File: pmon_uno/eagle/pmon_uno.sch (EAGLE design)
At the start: 42 parts, among them J1 USB, J2 USB, Q1 16Mhz, U1 LTC2943, U2 FT232RL, U3 LT1764AEQ, U4 ATMEGA328TQFP32

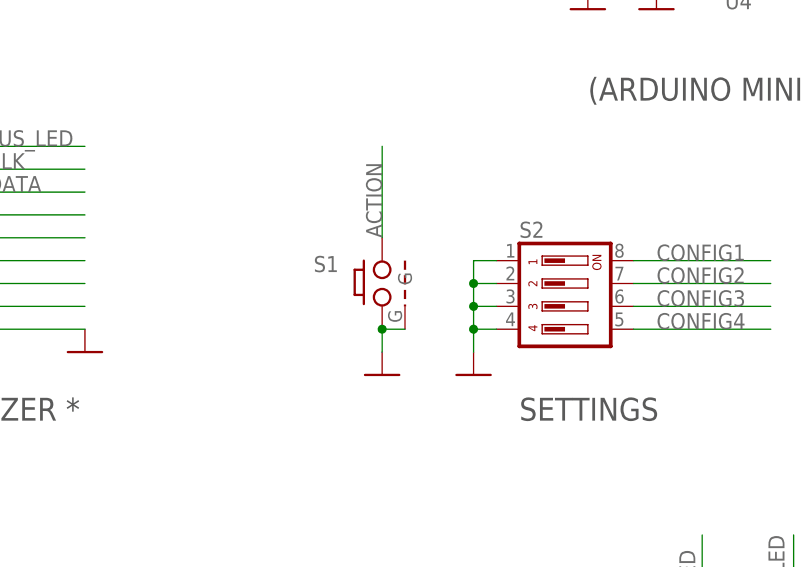
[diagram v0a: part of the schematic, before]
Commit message: Rev B is fully routed.
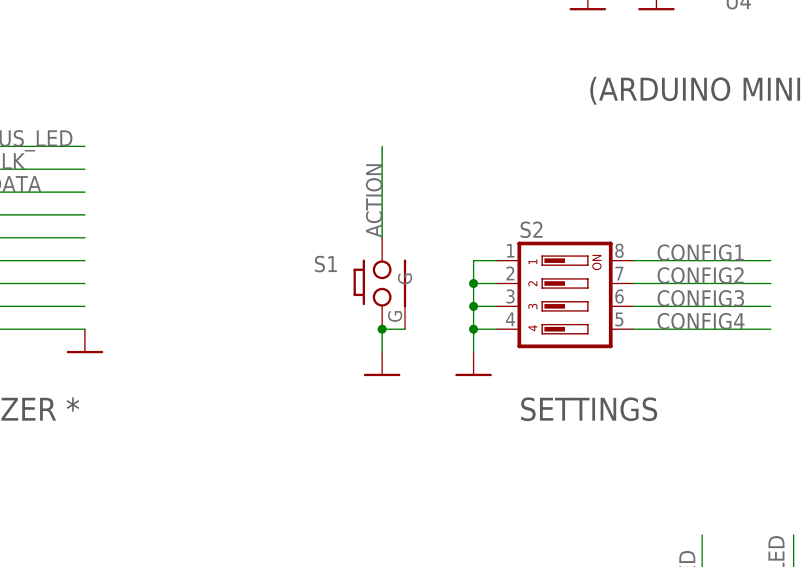
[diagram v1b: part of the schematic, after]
